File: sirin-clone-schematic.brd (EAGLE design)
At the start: 101.6 x 57.1 mm, 21 parts

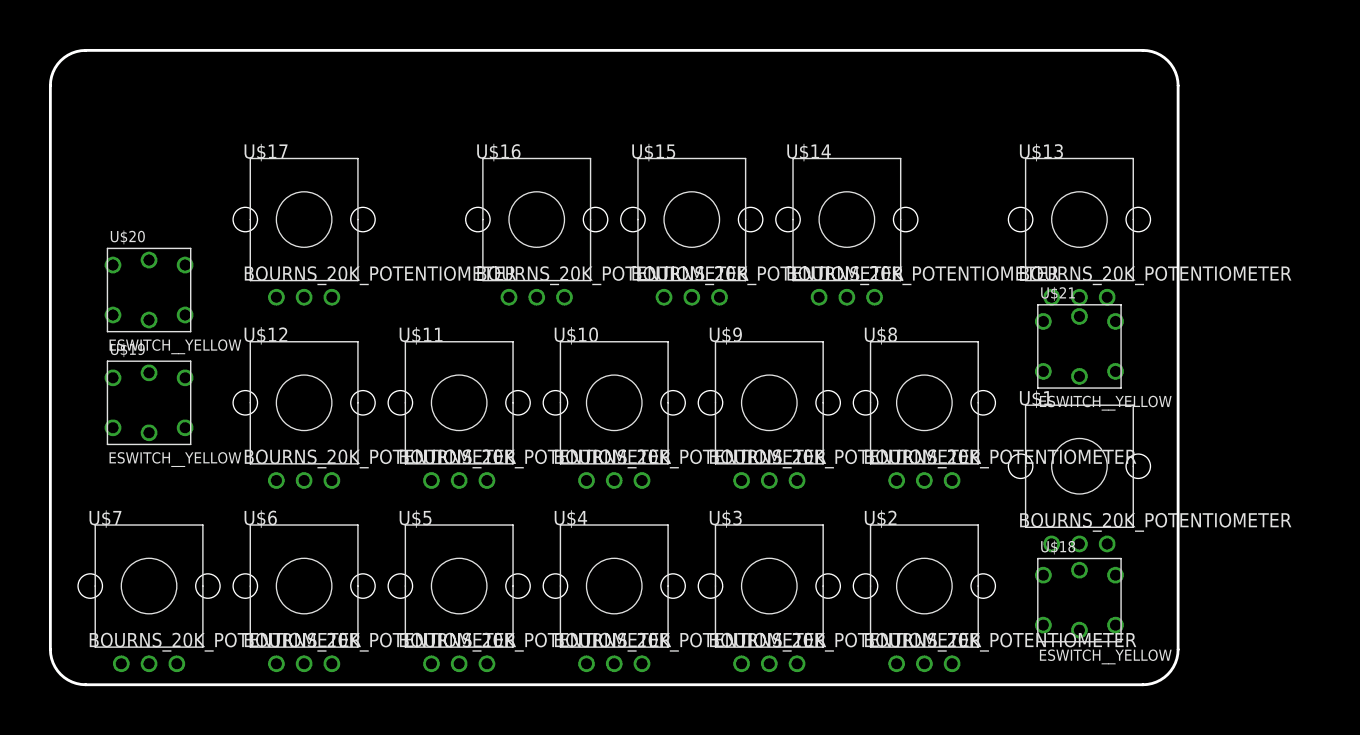
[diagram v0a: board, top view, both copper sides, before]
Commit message: lots o' routing
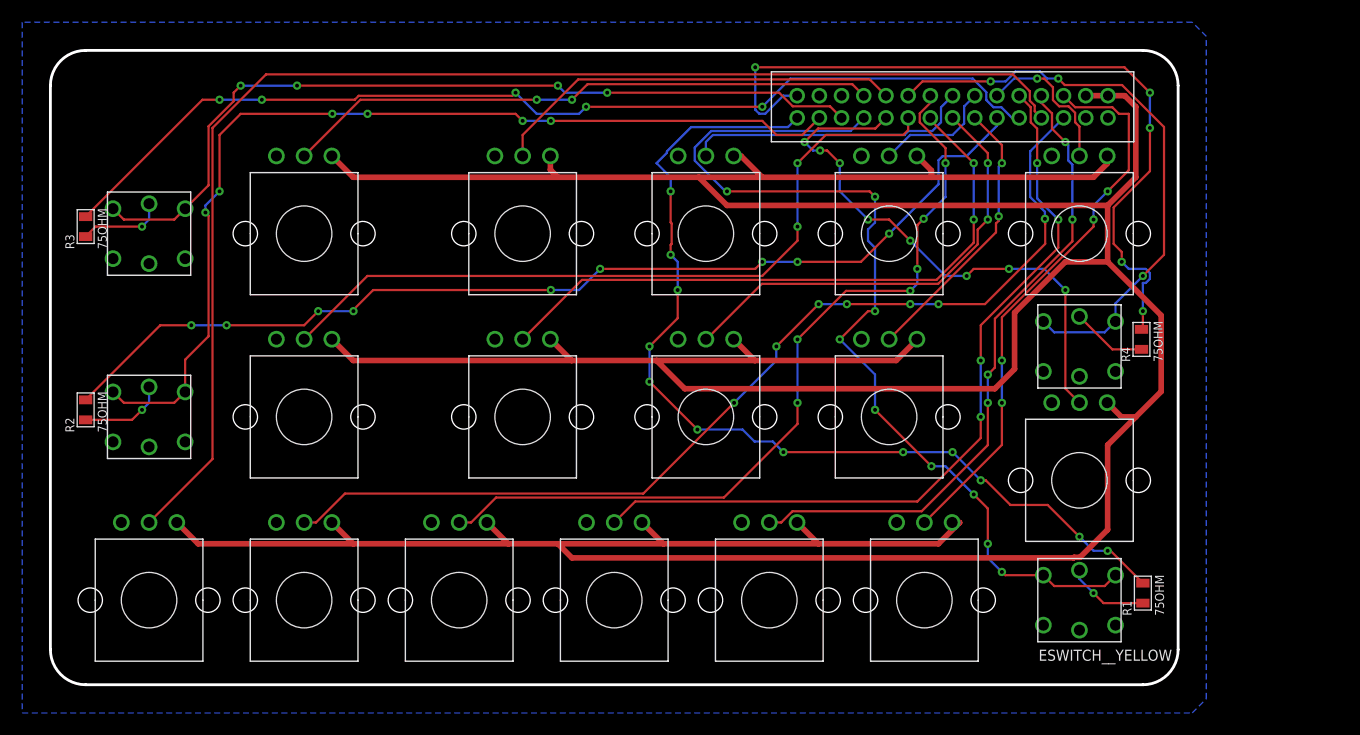
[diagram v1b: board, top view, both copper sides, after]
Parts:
- removed U$11: BOURNS_20K_POTENTIOMETER, sirin-clone-library:BOURNS_PTV09
- added J1: 30_PIN_CONNECTOR_MALE, sirin-clone-library:MOLEX_30PINCONNECTOR_2MM
- added R1, R2, R3, R4: 75OHM, sirin-clone-library:0805
- moved U$8 57.9 mm to (22.9, 40.6), turned to 180 degrees
- moved U$14 52.0 mm to (22.9, 24.1), turned to 180 degrees
- moved U$3 42.3 mm to (92.7, 40.6), turned to 180 degrees
- moved U$15 42.1 mm to (92.7, 18.4), turned to 180 degrees
- moved U$5 41.9 mm to (78.7, 7.62), turned to 180 degrees
- moved U$1 39.6 mm to (59.1, 40.6), turned to 180 degrees
- moved U$12 36.2 mm to (59.1, 24.1), turned to 180 degrees
- moved U$16 35.0 mm to (36.8, 7.62), turned to 180 degrees
- moved U$10 29.1 mm to (75.6, 40.6), turned to 180 degrees
- moved U$2 28.0 mm to (50.8, 7.62), turned to 180 degrees
- moved U$9 26.9 mm to (42.5, 40.6), turned to 180 degrees
- moved U$17 26.5 mm to (42.5, 24.1), turned to 180 degrees
- moved U$13 24.7 mm to (75.6, 24.1), turned to 180 degrees
- moved U$4 14.0 mm to (64.8, 7.62), turned to 180 degrees
- moved U$20 5.08 mm to (8.89, 40.6)
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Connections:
- new net 3.3V: J1.P$14, J1.P$15, U$1.1, U$10.1, U$12.1, U$13.1, U$14.1, U$15.1, U$16.1, U$17.1, U$2.1, U$3.1, U$4.1, U$5.1, U$6.1, U$7.1, U$8.1, U$9.1
- new net GND: J1.P$29, J1.P$30, U$1.3, U$10.3, U$12.3, U$13.3, U$14.3, U$15.3, U$16.3, U$17.3, U$18.-, U$18.1, U$18.2, U$19.-, U$19.1, U$19.2, U$2.3, U$20.-, U$20.1, U$20.2, U$21.-, U$21.1, U$21.2, U$3.3, U$4.3, U$5.3, U$6.3, U$7.3, U$8.3, U$9.3
- new net N$1: R1.1, U$18.+
- new net N$2: R2.1, U$19.+
- new net N$3: R3.1, U$20.+
- new net N$4: R4.1, U$21.+
- new net PIN15/KNOB1(VOL): J1.P$24, U$13.2
- new net PIN16/KNOB2: J1.P$28, U$6.2
- new net PIN17/KNOB3: J1.P$27, U$7.2
- new net PIN2/SW1: J1.P$19, U$18.3, U$18.4
- new net PIN20/KNOB4: J1.P$4, U$8.2
- new net PIN21/KNOB5: J1.P$5, U$9.2
- new net PIN24/LED1: J1.P$16, R1.2
- new net PIN25/LED2: J1.P$25, R2.2
- new net PIN26/KNOB6: J1.P$9, U$10.2
- new net PIN27/KNOB7: J1.P$22, U$17.2
- new net PIN28/KNOB8: J1.P$23, U$12.2
- new net PIN29/KNOB9: J1.P$21, U$14.2
- new net PIN3/SW2: J1.P$17, U$19.3, U$19.4
- new net PIN30/KNOB10: J1.P$20, U$15.2
- new net PIN31/KNOB11: J1.P$8, U$1.2
- new net PIN32/LED3: J1.P$26, R3.2
- new net PIN33/LED4: J1.P$1, R4.2
- new net PIN4/SW3: J1.P$18, U$20.3, U$20.4
- new net PIN5/SW4: J1.P$6, U$21.3, U$21.4
- new net PIN8/MIDILED: J1.P$3
- new net PINA10/KNOB12: J1.P$11, U$2.2
- new net PINA11/KNOB13: J1.P$10, U$3.2
- new net PINA12/KNOB14: J1.P$12, U$4.2
- new net PINA13/KNOB15: J1.P$13, U$5.2
- new net PINA14/KNOB16: J1.P$7, U$16.2
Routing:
- net 3.3V: track 0.00 -> 412.9 mm
- net PIN17/KNOB3: track 0.00 -> 117.0 mm
- net PIN25/LED2: track 0.00 -> 94.4 mm, vias 0 -> 9
- net PIN32/LED3: track 0.00 -> 92.7 mm, vias 0 -> 5
- net PIN16/KNOB2: track 0.00 -> 91.1 mm, vias 0 -> 7
- net PIN2/SW1: track 0.00 -> 89.1 mm, vias 0 -> 9
- net PIN3/SW2: track 0.00 -> 88.2 mm, vias 0 -> 6
- net PIN24/LED1: track 0.00 -> 88.0 mm, vias 0 -> 12
- net PIN4/SW3: track 0.00 -> 75.8 mm, vias 0 -> 4
- net PINA14/KNOB16: track 0.00 -> 74.0 mm, vias 0 -> 6
- net PINA10/KNOB12: track 0.00 -> 71.4 mm, vias 0 -> 4
- net PIN33/LED4: track 0.00 -> 70.3 mm, vias 0 -> 5
- net PIN29/KNOB9: track 0.00 -> 67.4 mm, vias 0 -> 2
- net PINA12/KNOB14: track 0.00 -> 58.4 mm, vias 0 -> 4
- net PIN27/KNOB7: track 0.00 -> 57.1 mm, vias 0 -> 2
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- added copper zone on layer 16, net GND
